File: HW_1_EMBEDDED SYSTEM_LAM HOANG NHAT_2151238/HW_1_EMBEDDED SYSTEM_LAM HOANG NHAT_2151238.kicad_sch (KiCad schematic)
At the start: 17 parts

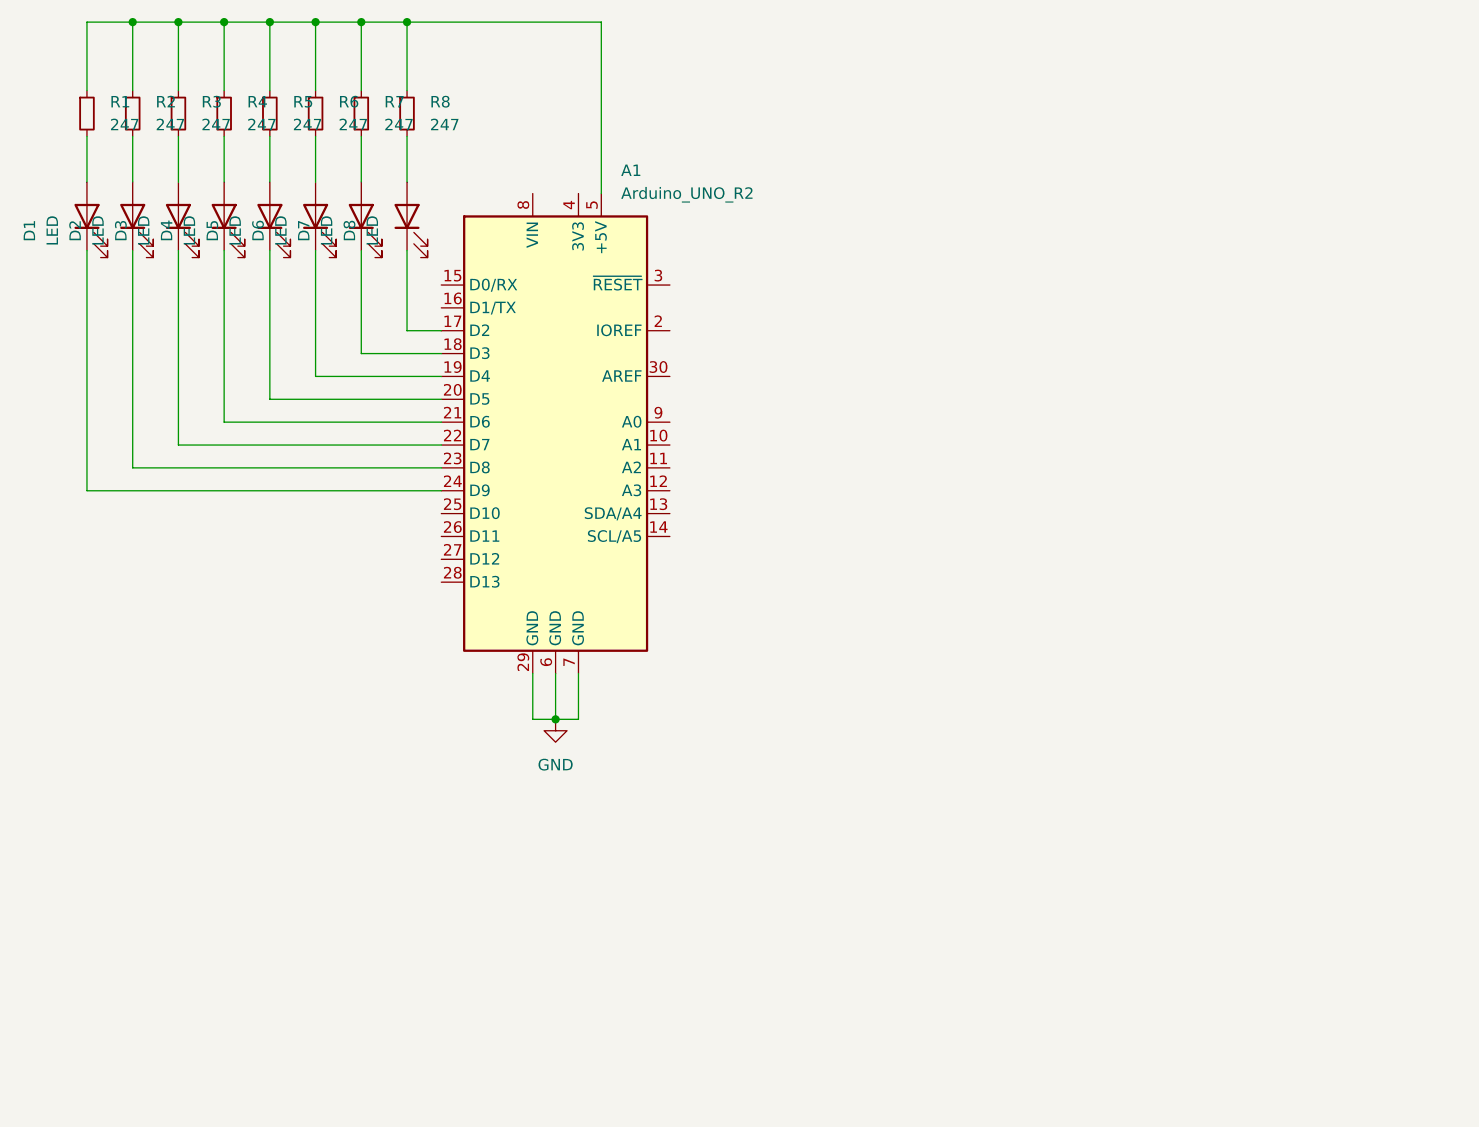
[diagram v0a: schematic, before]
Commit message: Add files via upload
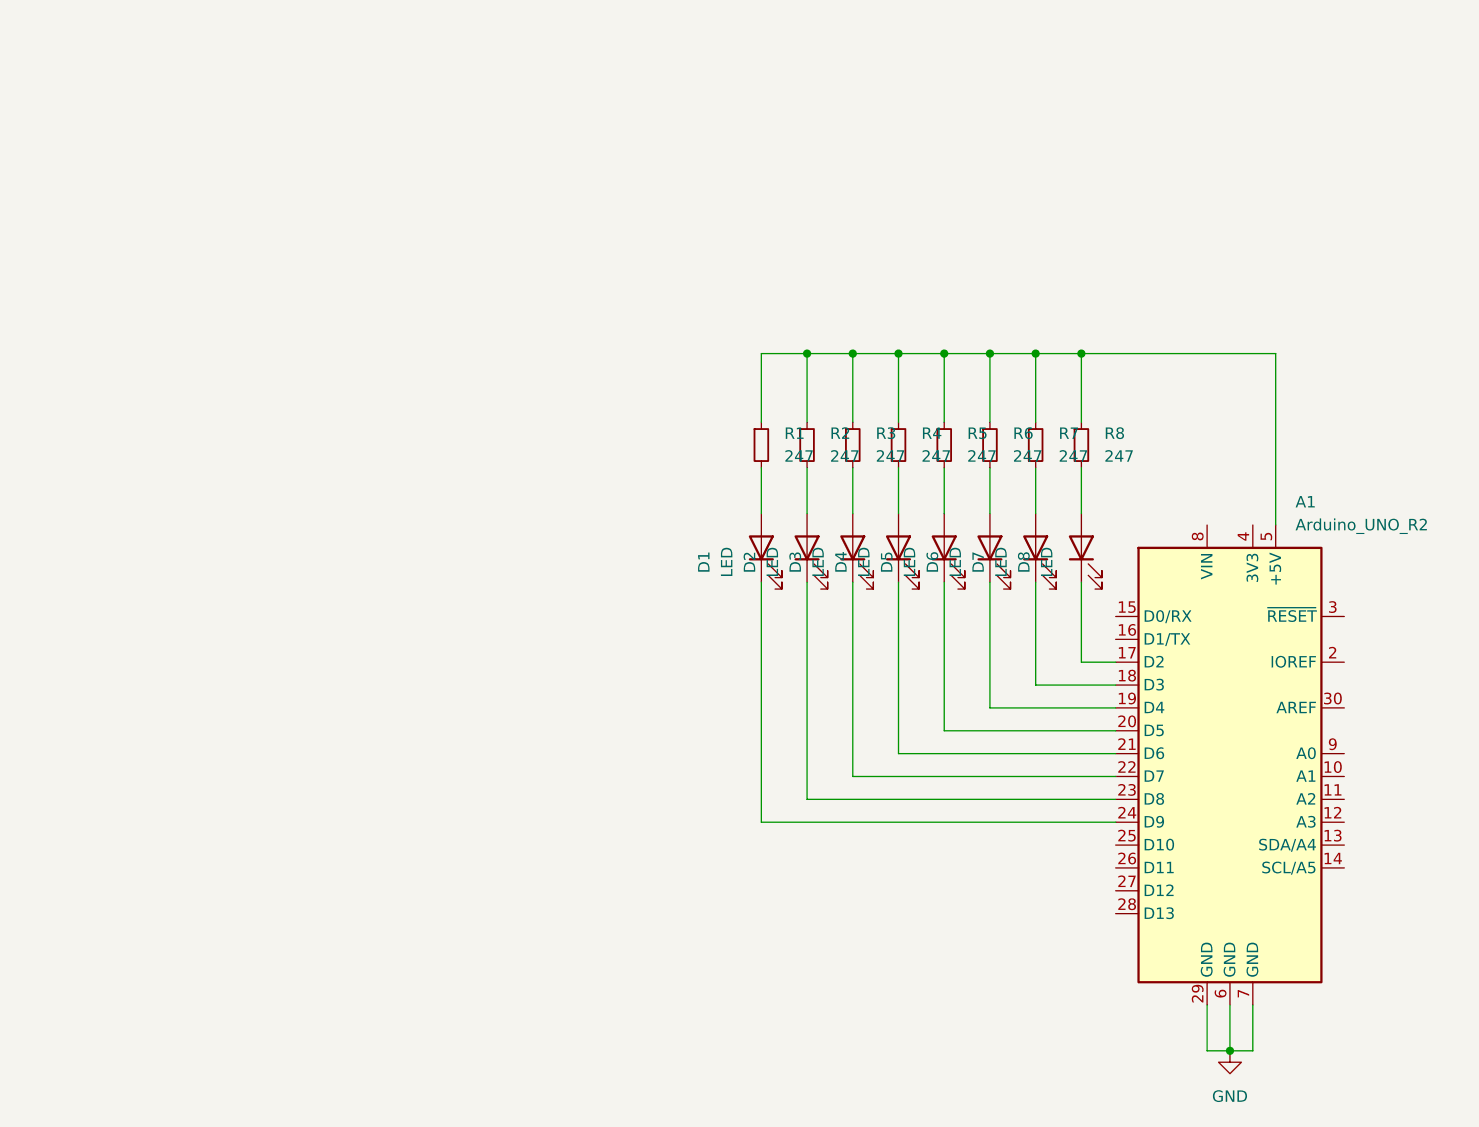
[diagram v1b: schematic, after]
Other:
- moved on the sheet: A1, D1, D2, D3, D4, D5, D6, D7, D8, R1, R2, R3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
